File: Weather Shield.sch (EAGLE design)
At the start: 38 parts, among them Q1 BSS138, Q2 BSS138, U1 DS3231SN, U4 MPL3115A2LGA8, U5 HTU21D

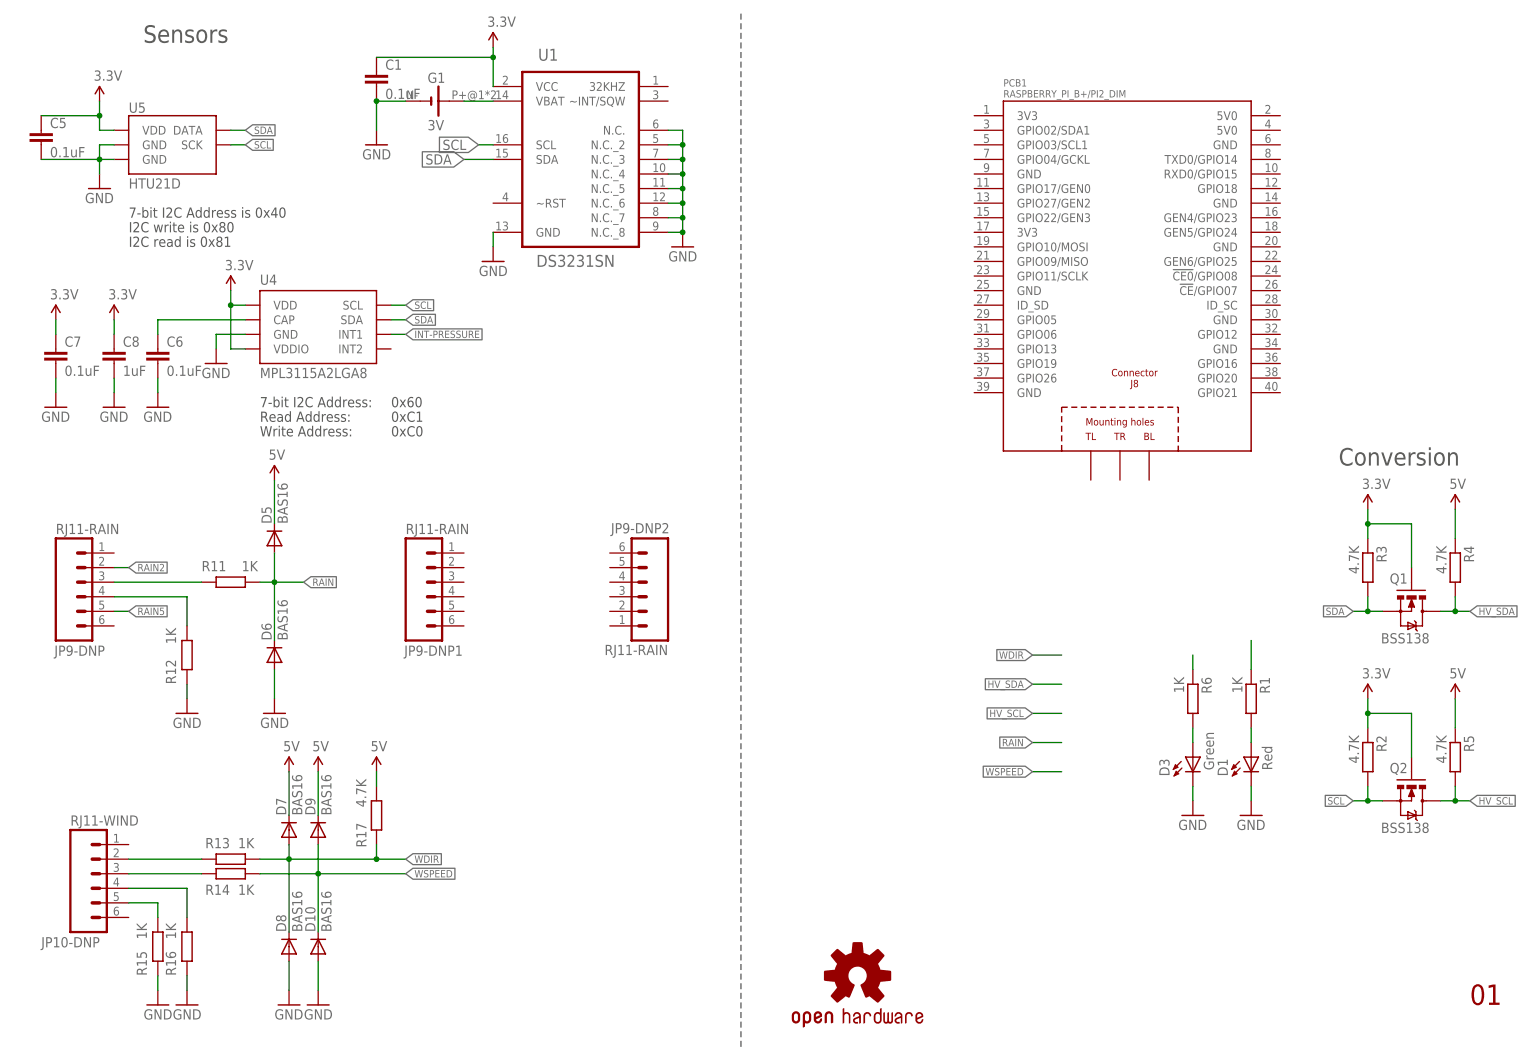
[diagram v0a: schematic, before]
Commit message: initial project version
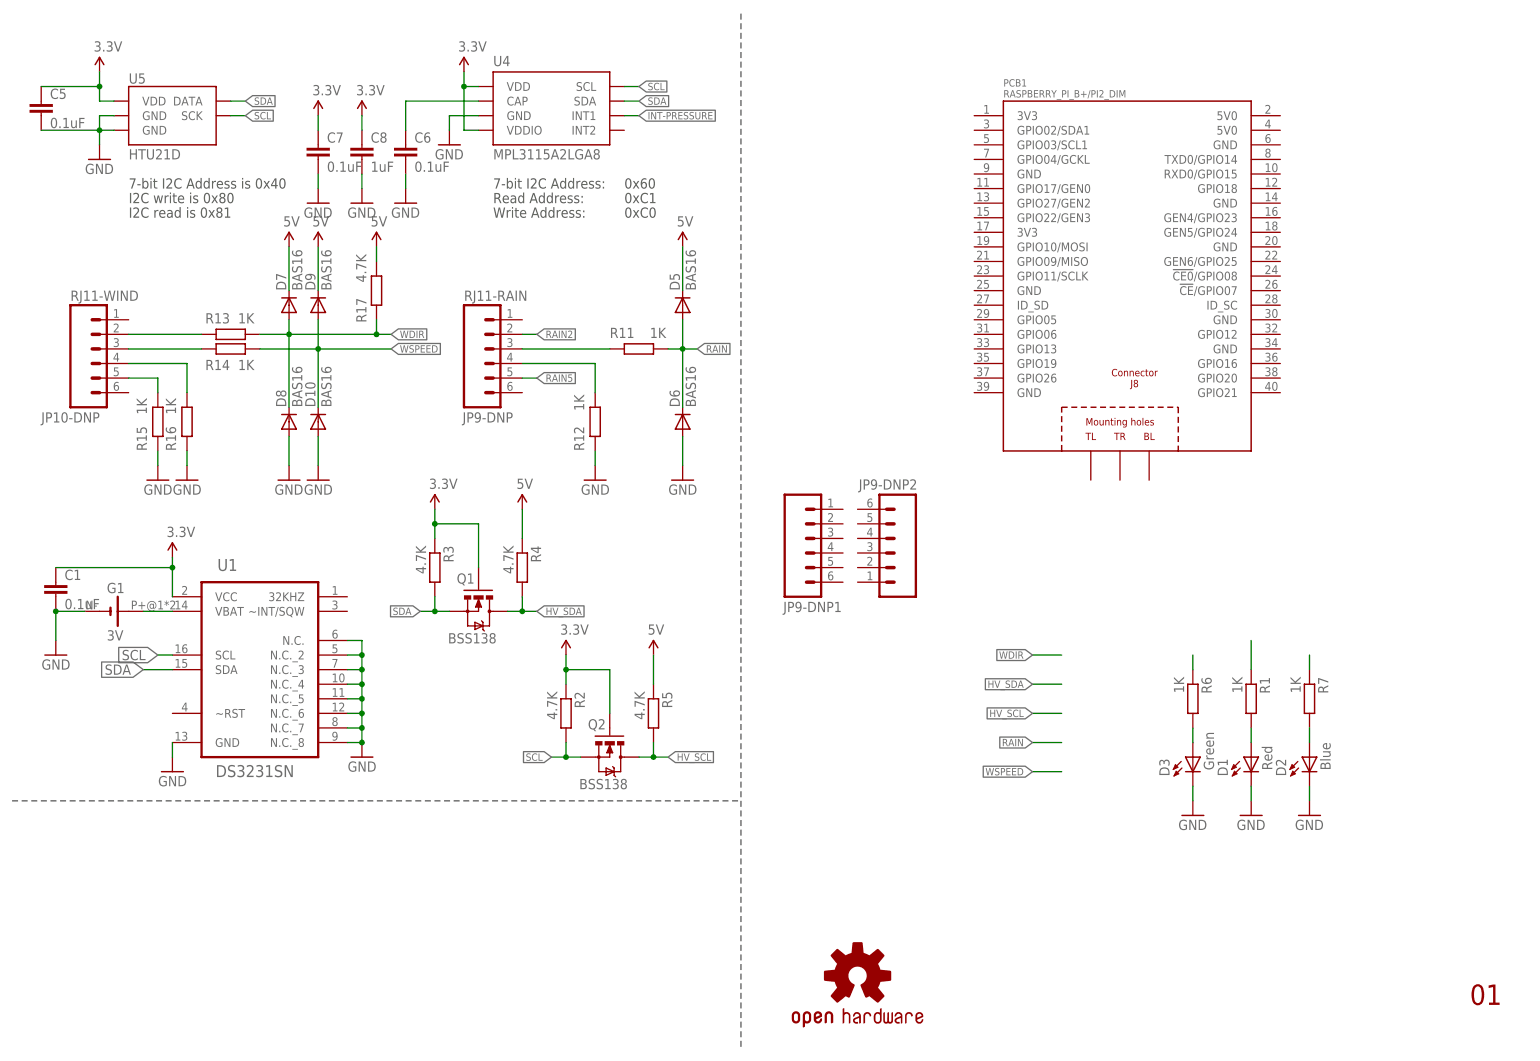
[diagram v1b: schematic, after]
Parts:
- added D2: Blue, SparkFun:LED0603
- added R7: 1K, rcl:R-EU_R0603
- JP9-DNP1, JP9-DNP2: value RJ11-RAIN -> RJ11-6PTH
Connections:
- new net N$10: D2.A, R7.2
- new net STAT3: R7.1
- net GND: now also D2.C
- net SCL: now also U1.SCL
- net SDA: now also U1.SDA
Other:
- note added: "RTC Clock"
- note removed: "Conversion"
- note removed: "Sensors"
- moved on the sheet: C1, C5, C6, C7, C8, D10, D5, D6, D7, D8, D9, G1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
